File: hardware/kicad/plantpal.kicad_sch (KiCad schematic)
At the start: 0 parts

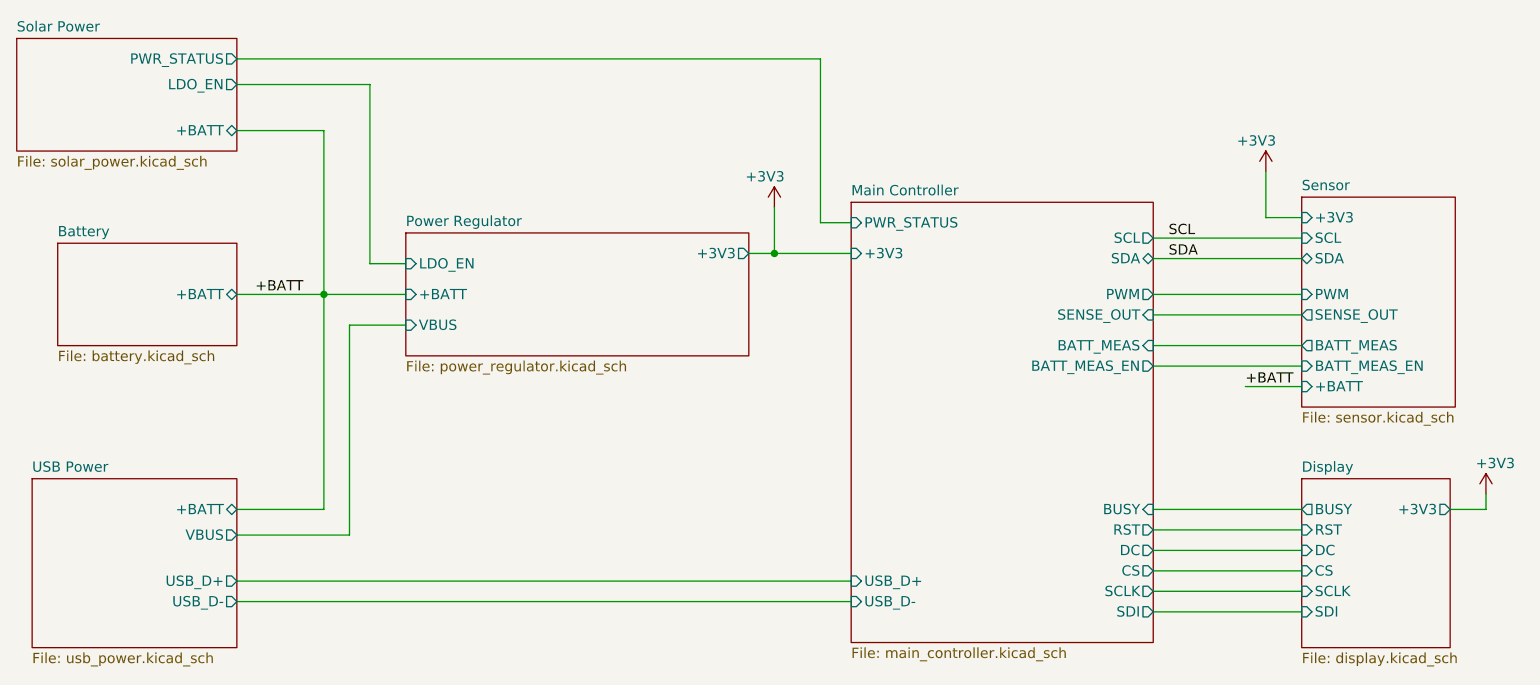
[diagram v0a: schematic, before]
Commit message: wip: revision 2
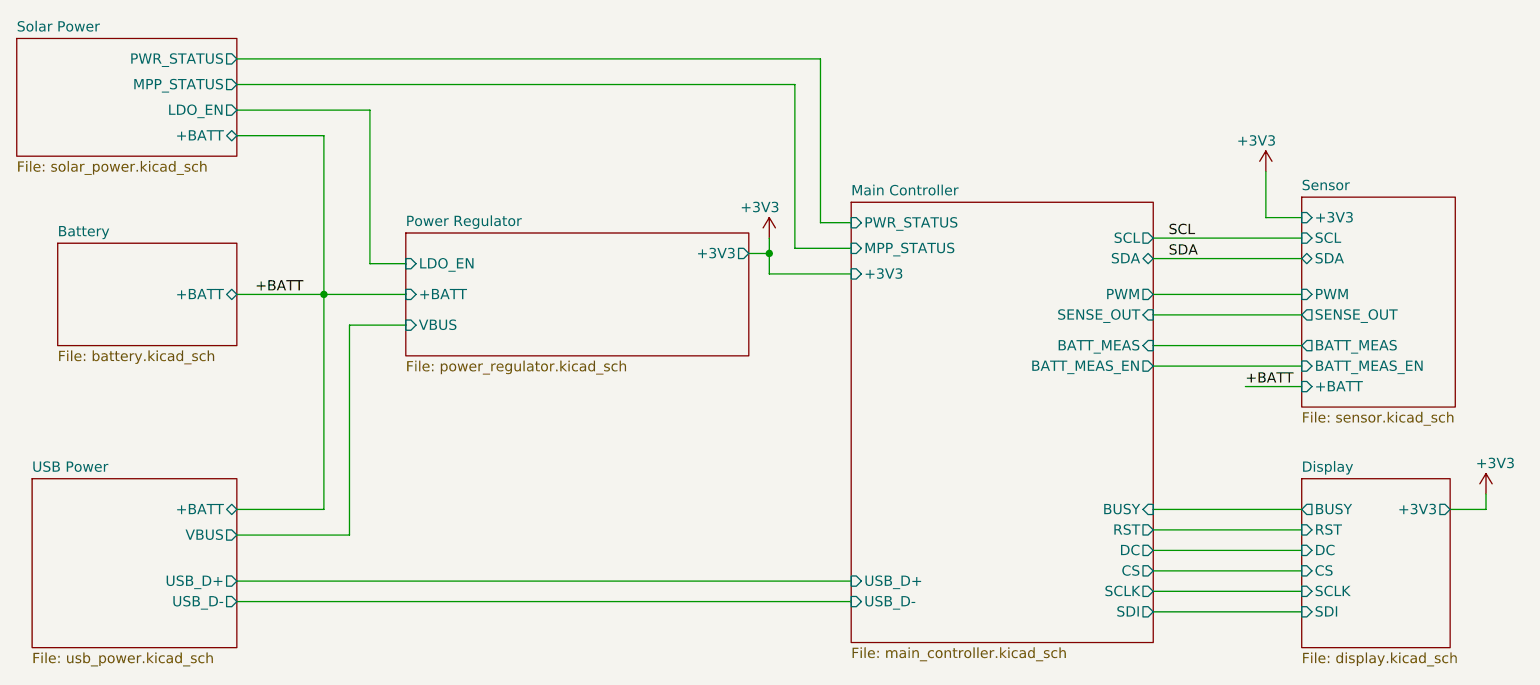
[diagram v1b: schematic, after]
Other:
- sheet Main Controller ports: added MPP_STATUS; removed none
- sheet Solar Power ports: added MPP_STATUS; removed none
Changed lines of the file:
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@@
     (rev "2")
   )
-  (junction (at 149.225 77.47) (diameter 0) (color 0 0 0 0)
+  (junction (at 148.59 77.47) (diameter 0) (color 0 0 0 0)
   )
   (junction (at 93.345 82.55) (diameter 0) (color 0 0 0 0)
   )
-  (wire (pts (xy 149.225 77.47) (xy 158.75 77.47))
+  (wire (pts (xy 148.59 77.47) (xy 146.05 77.47))
+    (stroke (width 0) (type default))
+  )
+  (wire (pts (xy 93.345 62.865) (xy 93.345 82.55))
     (stroke (width 0) (type default))
   )
@@
     (stroke (width 0) (type default))
   )
+  (wire (pts (xy 151.765 56.515) (xy 151.765 76.835))
+    (stroke (width 0) (type default))
+  )
   (wire (pts (xy 196.215 111.76) (xy 214.63 111.76))
     (stroke (width 0) (type default))
   )
+  (wire (pts (xy 158.75 80.01) (xy 148.59 80.01))
+    (stroke (width 0) (type default))
+  )
+  (wire (pts (xy 148.59 77.47) (xy 148.59 75.565))
+    (stroke (width 0) (type default))
+  )
   (wire (pts (xy 214.63 73.025) (xy 210.185 73.025))
     (stroke (width 0) (type default))
@@
     (stroke (width 0) (type default))
   )
-  (wire (pts (xy 99.06 56.515) (xy 99.06 78.74))
-    (stroke (width 0) (type default))
-  )
   (wire (pts (xy 154.94 73.66) (xy 158.75 73.66))
     (stroke (width 0) (type default))
@@
     (stroke (width 0) (type default))
   )
-  (wire (pts (xy 93.345 62.23) (xy 93.345 82.55))
-    (stroke (width 0) (type default))
-  )
   (wire (pts (xy 196.215 82.55) (xy 214.63 82.55))
     (stroke (width 0) (type default))
@@
     (stroke (width 0) (type default))
   )
+  (wire (pts (xy 151.765 76.835) (xy 158.75 76.835))
+    (stroke (width 0) (type default))
+  )
   (wire (pts (xy 99.06 78.74) (xy 103.505 78.74))
     (stroke (width 0) (type default))
   )
-  (wire (pts (xy 82.55 62.23) (xy 93.345 62.23))
-    (stroke (width 0) (type default))
-  )
   (wire (pts (xy 82.55 53.34) (xy 154.94 53.34))
     (stroke (width 0) (type default))
@@
     (stroke (width 0) (type default))
   )
+  (wire (pts (xy 99.06 59.69) (xy 99.06 78.74))
+    (stroke (width 0) (type default))
+  )
+  (wire (pts (xy 148.59 80.01) (xy 148.59 77.47))
+    (stroke (width 0) (type default))
+  )
   (wire (pts (xy 196.215 91.44) (xy 214.63 91.44))
     (stroke (width 0) (type default))
@@
     (stroke (width 0) (type default))
   )
-  (wire (pts (xy 146.05 77.47) (xy 149.225 77.47))
-    (stroke (width 0) (type default))
-  )
-  (wire (pts (xy 149.225 71.755) (xy 149.225 77.47))
-    (stroke (width 0) (type default))
-  )
-  (wire (pts (xy 82.55 56.515) (xy 99.06 56.515))
+  (wire (pts (xy 82.55 56.515) (xy 151.765 56.515))
+    (stroke (width 0) (type default))
+  )
+  (wire (pts (xy 82.55 62.865) (xy 93.345 62.865))
+    (stroke (width 0) (type default))
+  )
+  (wire (pts (xy 82.55 59.69) (xy 99.06 59.69))
     (stroke (width 0) (type default))
   )
@@
     )
   )
-  (symbol (lib_id "power:+3V3") (at 149.225 71.755 0) (unit 1)
+  (symbol (lib_id "power:+3V3") (at 148.59 75.565 0) (unit 1)
     (in_bom yes) (on_board yes) (dnp no)
-    (property "Reference" "#PWR01" (at 149.225 75.565 0)
-      (effects (font (size 1.27 1.27)) hide)
-    )
-    (property "Value" "+3V3" (at 150.495 67.945 0)
-      (effects (font (size 1.27 1.27)) (justify right))
-    )
-    (property "Footprint" "" (at 149.225 71.755 0)
-      (effects (font (size 1.27 1.27)) hide)
-    )
-    (property "Datasheet" "" (at 149.225 71.755 0)
+    (property "Reference" "#PWR062" (at 148.59 79.375 0)
+      (effects (font (size 1.27 1.27)) hide)
+    )
+    (property "Value" "+3V3" (at 149.86 71.755 0)
+      (effects (font (size 1.27 1.27)) (justify right))
+    )
+    (property "Footprint" "" (at 148.59 75.565 0)
+      (effects (font (size 1.27 1.27)) hide)
+    )
+    (property "Datasheet" "" (at 148.59 75.565 0)
       (effects (font (size 1.27 1.27)) hide)
     )
@@
       (project "plantpal"
         (path "/59b4123e-c7be-466b-a5db-658b8f0c1171"
-          (reference "#PWR01") (unit 1)
+          (reference "#PWR062") (unit 1)
         )
         (path "/59b4123e-c7be-466b-a5db-658b8f0c1171/416559aa-55f3-4db2-bf13-04c2bb6b0caa"
@@
     )
   )
-  (sheet (at 55.245 50.8) (size 27.305 13.97) (fields_autoplaced)
+  (sheet (at 55.245 50.8) (size 27.305 14.605) (fields_autoplaced)
     (stroke (width 0.1524) (type solid))
     (fill (color 0 0 0 0.0000))
@@
       (effects (font (size 1.27 1.27)) (justify left bottom))
     )
-    (property "Sheetfile" "solar_power.kicad_sch" (at 55.245 65.3546 0)
-      (effects (font (size 1.27 1.27)) (justify left top))
-    )
-    (pin "LDO_EN" output (at 82.55 56.515 0)
+    (property "Sheetfile" "solar_power.kicad_sch" (at 55.245 65.9896 0)
+      (effects (font (size 1.27 1.27)) (justify left top))
+    )
+    (pin "LDO_EN" output (at 82.55 59.69 0)
       (effects (font (size 1.27 1.27)) (justify right))
     )
@@
       (effects (font (size 1.27 1.27)) (justify right))
     )
-    (pin "+BATT" bidirectional (at 82.55 62.23 0)
+    (pin "+BATT" bidirectional (at 82.55 62.865 0)
+      (effects (font (size 1.27 1.27)) (justify right))
+    )
+    (pin "MPP_STATUS" output (at 82.55 56.515 0)
       (effects (font (size 1.27 1.27)) (justify right))
     )
@@
       (effects (font (size 1.27 1.27)) (justify left))
     )
-    (pin "+3V3" input (at 158.75 77.47 180)
+    (pin "+3V3" input (at 158.75 80.01 180)
       (effects (font (size 1.27 1.27)) (justify left))
     )
@@
       (effects (font (size 1.27 1.27)) (justify right))
     )
-    (instances
+    (pin "MPP_STATUS" input (at 158.75 76.835 180)
+      (effects (font (size 1.27 1.27)) (justify left))
+    )
+    (instances
